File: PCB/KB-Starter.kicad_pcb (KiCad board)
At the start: 2 copper layers, 100.1 x 104.6 mm, 69 parts, among them J1 USB_C_Receptacle_USB2.0, J2 SWD, SW1 SW_Push, U1 W25Q128JVS, U2 USBLC6-2SC6, U3 XC6206PxxxMR, U5 RP2040, Y1 12MHz

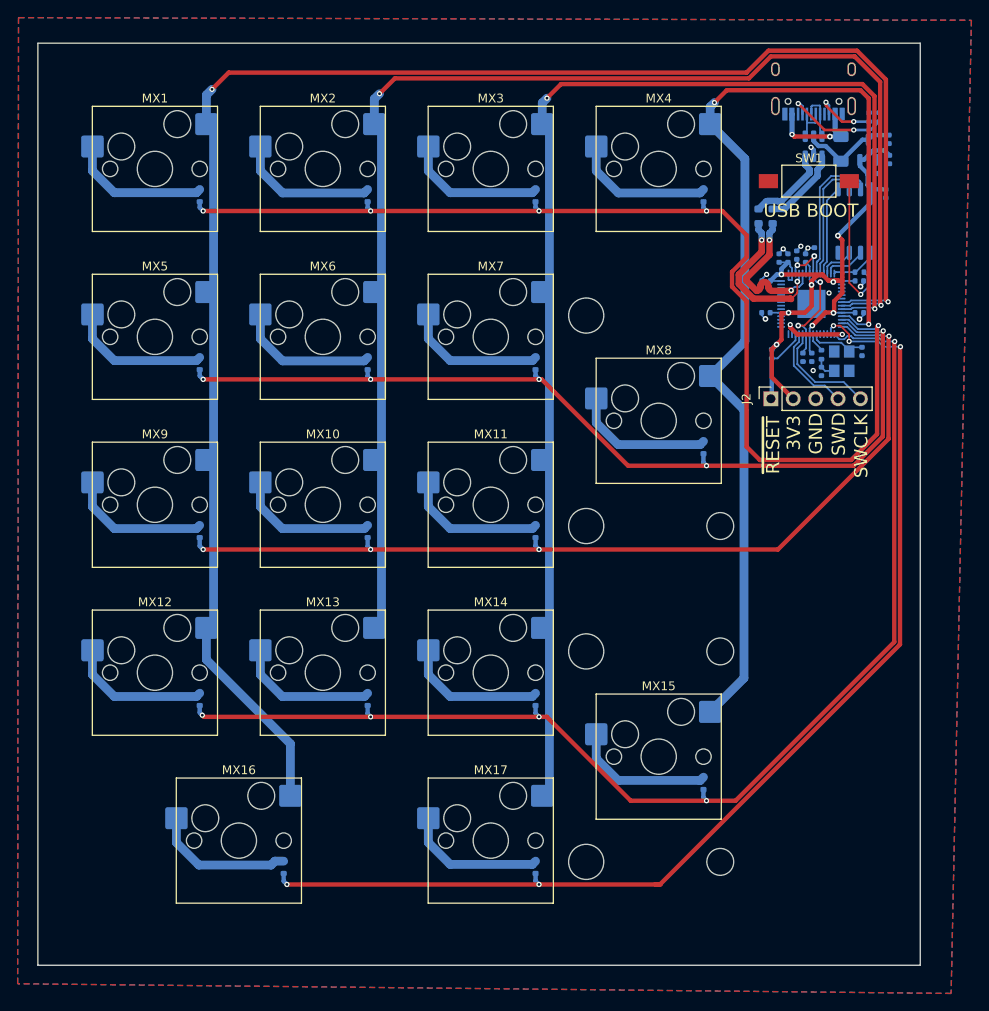
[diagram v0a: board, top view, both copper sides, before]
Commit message: add missing 3d models, cleanup for KiCad 8, swd
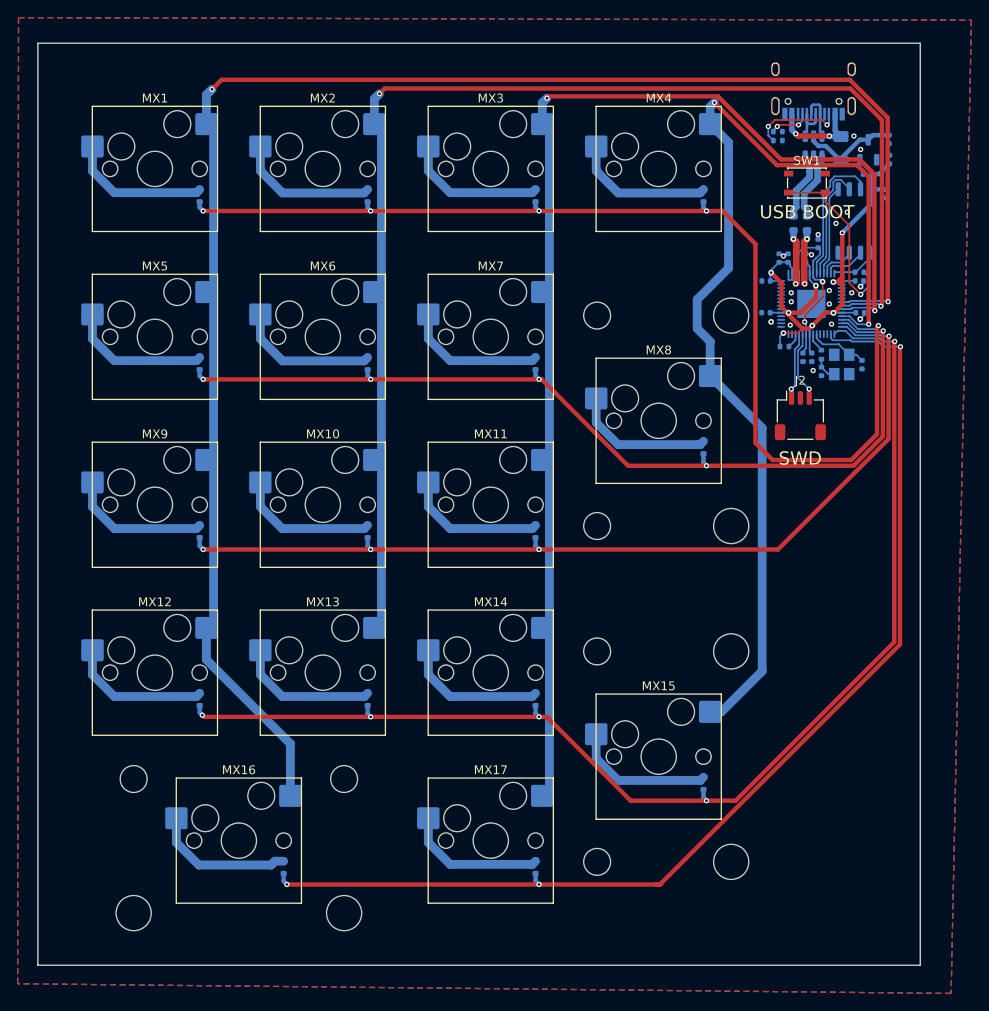
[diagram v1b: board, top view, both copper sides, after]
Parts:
- added STAB1: Stabilizer_Cherry_MX_2.00u, PCM_Mounting_Keyboard_Stabilizer:Stabilizer_Cherry_MX_2.00u, F.Cu at (43.0, 110.7)
- J2: value SWD -> 3-pin SWD; footprint Connector_PinSocket_2.54mm:PinSocket_1x05_P2.54mm_Vertical -> Connector_JST:JST_SH_SM03B-SRSS-TB_1x03-1MP_P1.00mm_Horizontal
- MX1, MX10, MX11, MX13, MX14, MX17, MX2, MX3, MX4, MX5, MX6, MX7, MX9: value SW_Push -> Kailh Hotswap
- MX12, MX15, MX8: value SW_Push -> Kailh Hotswap; footprint PCM_Switch_Keyboard_Hotswap_Kailh:SW_Hotswap_Kailh_MX_2.00u_90deg -> PCM_Switch_Keyboard_Hotswap_Kailh:SW_Hotswap_Kailh_MX_1.00u
- MX16: value SW_Push -> Kailh Hotswap; footprint PCM_Switch_Keyboard_Hotswap_Kailh:SW_Hotswap_Kailh_MX_2.00u -> PCM_Switch_Keyboard_Hotswap_Kailh:SW_Hotswap_Kailh_MX_1.00u
- SW1: footprint Button_Switch_SMD:SW_SPST_FSMSM -> Button_Switch_SMD:SW_SPST_PTS810
- moved R3 11.6 mm to (104.1, 30.2), turned to 0 degrees
- moved R4 10.7 mm to (104.1, 31.2), turned to 0 degrees
- moved R6 4.05 mm to (105.9, 40.6)
- moved R5 3.97 mm to (107.4, 40.6)
- moved J2 3.86 mm to (106.7, 62.5), turned to 0 degrees
- moved R2 1.68 mm to (104.9, 54.6), turned to 0 degrees
- moved C2 1.50 mm to (113.7, 56.7)
- moved C5 1.04 mm to (108.7, 42.9)
- moved C4 0.55 mm to (106.3, 43.7)
- moved C17 0.50 mm to (114.3, 35.1), turned to 0 degrees
- moved Y1 0.37 mm to (111.4, 56.6)
- moved SW1 0.31 mm to (107.4, 36.1)
- moved C13 0.08 mm to (113.5, 50.8)
- turned C7 to 90 degrees
- turned STAB2 to 90 degrees
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- renumbered REF** to STAB2, REF** to STAB3
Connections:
- J2 pad 1: ~{RESET} -> SWD
- J2 pad 2: +3V3 -> GND
- J2 pad 3: GND -> SWCLK
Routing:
- net GND: track 15.2 -> 3.88 mm, vias 12 -> 18
- net +3V3: track 80.0 -> 69.5 mm
- net USBD_N: track 18.0 -> 7.50 mm
- net USBD_P: track 17.2 -> 7.45 mm
- net /CC1: track 12.3 -> 4.66 mm
- net ~{RESET}: track 8.86 -> 1.70 mm
- net COL3: track 148.5 -> 142.4 mm
- net COL2: track 152.6 -> 147.4 mm
- net COL1: track 196.7 -> 191.5 mm
- net SWCLK: track 12.4 -> 7.98 mm, vias 0 -> 1
- net COL4: track 123.3 -> 119.1 mm
- net /~{USB_BOOT}: track 16.5 -> 20.5 mm
- net /CC2: track 7.52 -> 10.3 mm
- net SWD: track 10.4 -> 7.62 mm, vias 0 -> 1
- net ROW1: track 126.7 -> 124.5 mm
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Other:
- board text removed: "3V3"
- board text removed: "GND"
- board text removed: "SWCLK"
- board text removed: "~{RESET}"
